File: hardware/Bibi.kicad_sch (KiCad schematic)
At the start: 14 parts, among them M1 Motor_Servo, M2 Motor_Servo, M3 Fan_3pin, U2 Left, U3 Right, U4 GP2Y0A51SK0F

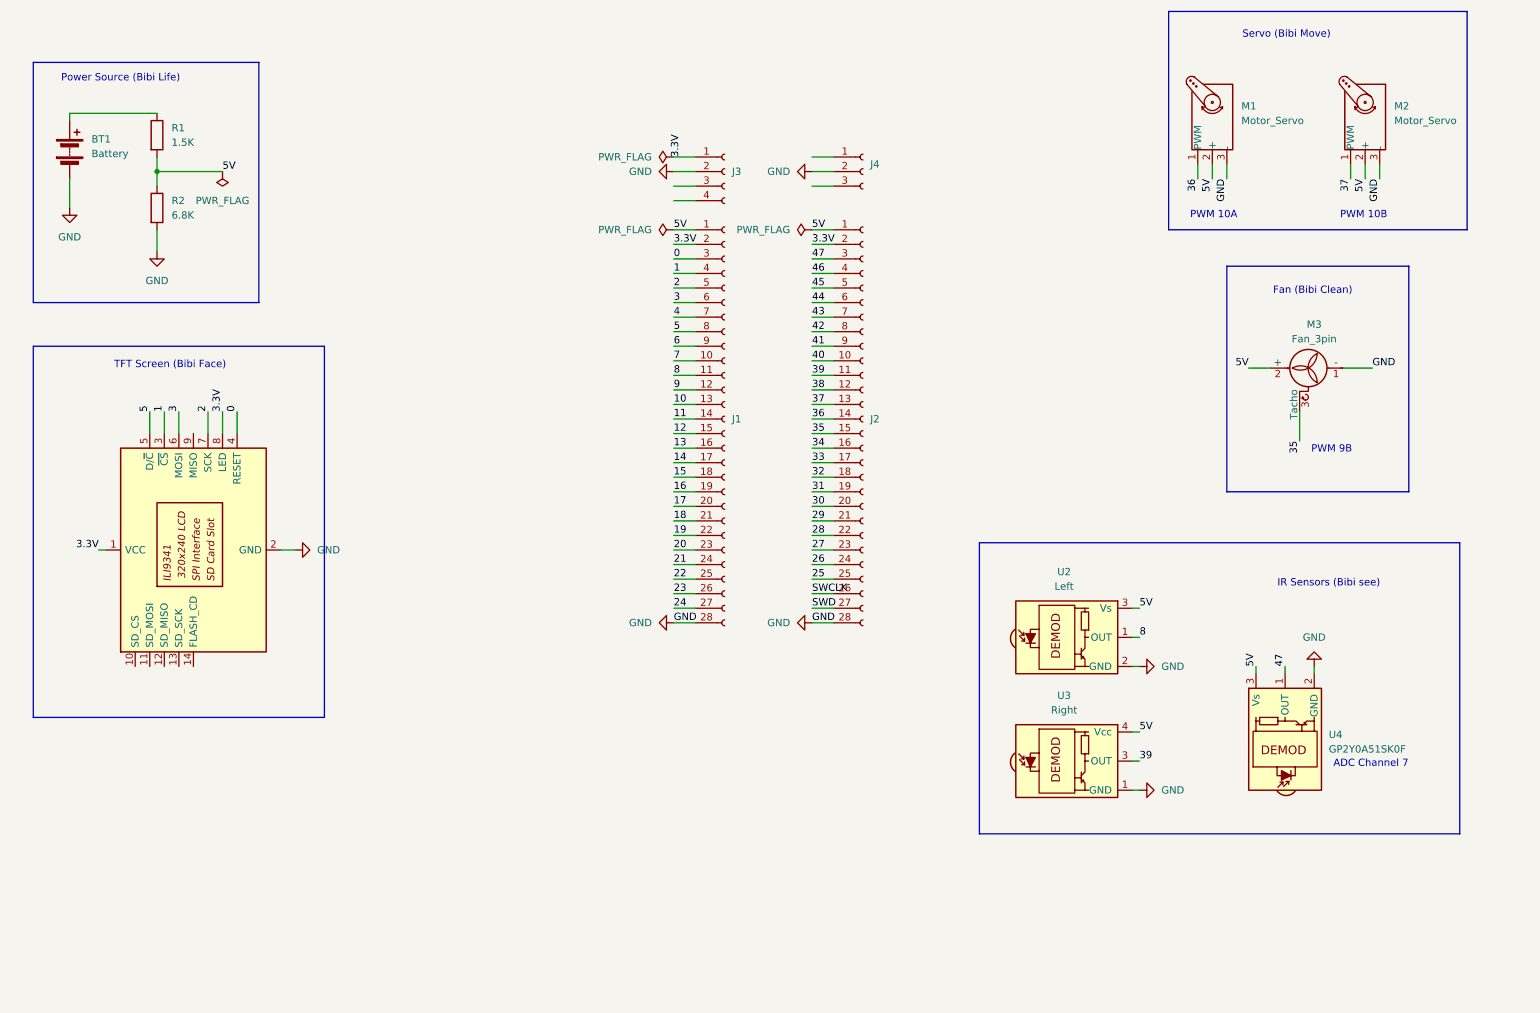
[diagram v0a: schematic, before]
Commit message: updated schematic
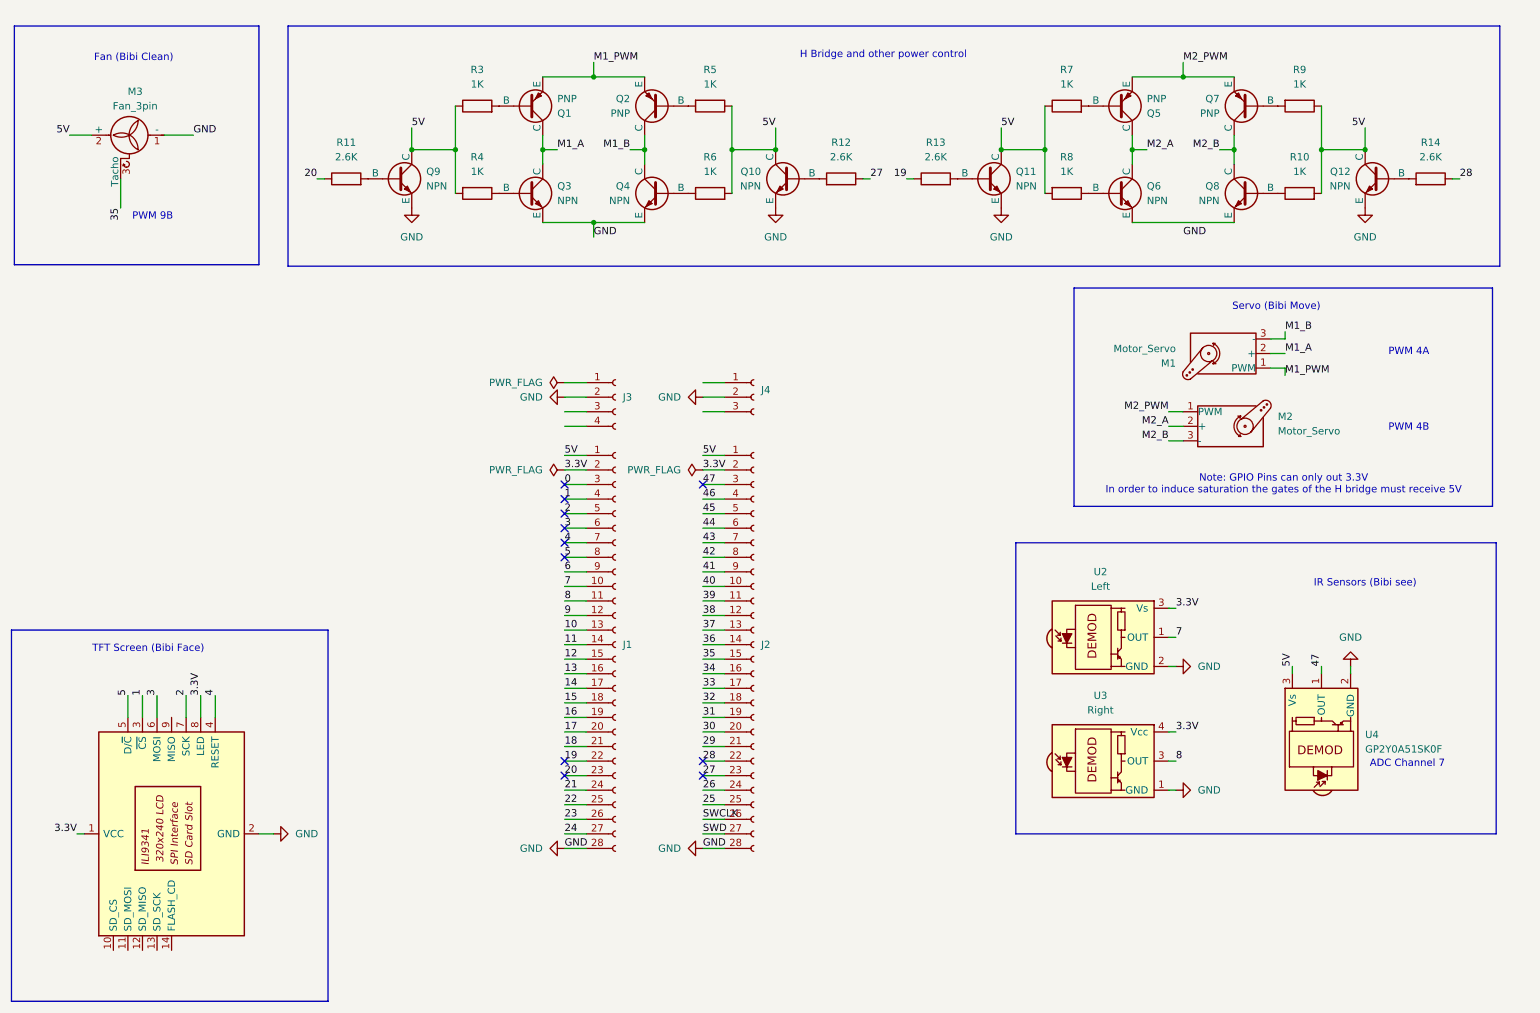
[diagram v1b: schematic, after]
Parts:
- removed BT1: Battery, symbol Device:Battery
- removed R1: 1.5K, Resistor_THT:R_Axial_DIN0411_L9.9mm_D3.6mm_P12.70mm_Horizontal, symbol Device:R
- removed R2: 6.8K, Resistor_THT:R_Axial_DIN0411_L9.9mm_D3.6mm_P12.70mm_Horizontal, symbol Device:R
- added Q1, Q2, Q5, Q7: PNP, symbol Simulation_SPICE:PNP
- added Q10, Q11, Q12, Q3, Q4, Q6, Q8, Q9: NPN, symbol Simulation_SPICE:NPN
- added R10, R3, R4, R5, R6, R7, R8, R9: 1K, symbol Device:R
- added R11, R12, R13, R14: 2.6K, symbol Device:R
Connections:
- net 0: no longer U1.4 (RESET)
- net 19: now also R13.1
- net 20: now also R11.1
- net 27: now also R12.1
- net 28: now also R14.1
- net 3.3V: now also U2.3 (Vs), U3.4 (Vcc); no longer J3.1 (Pin_1)
- net 36: no longer M1.1 (PWM)
- net 37: no longer M2.1 (PWM)
- net 39: no longer U3.3 (OUT)
- net 4: now also U1.4 (RESET)
- net 5V: now also Q10.1 (C), Q11.1 (C), Q12.1 (C), Q9.1 (C), R10.2, R3.1, R4.2, R5.1, R6.2, R7.1, R8.2, R9.1; no longer M1.2 (+), M2.2 (+), U2.3 (Vs), U3.4 (Vcc)
- net 7: now also U2.1 (OUT)
- net 8: now also U3.3 (OUT); no longer U2.1 (OUT)
- net GND: now also Q10.3 (E), Q11.3 (E), Q12.3 (E), Q3.3 (E), Q4.3 (E), Q9.3 (E); no longer M1.3 (-), M2.3 (-)
- new net: Q9.2 (B), R11.2
- new net: Q7.2 (B), R9.2
- new net: Q1.2 (B), R3.2
- new net: Q6.2 (B), R8.1
- new net: Q4.2 (B), R6.1
- new net: Q5.2 (B), R7.2
- new net: Q12.2 (B), R14.2
- new net: Q2.2 (B), R5.2
- new net: Q3.2 (B), R4.1
- new net: Q8.2 (B), R10.1
- new net: Q6.3 (E), Q8.3 (E)
- new net: Q10.2 (B), R12.2
- new net: Q11.2 (B), R13.2
- new net M1_A: M1.2 (+), Q1.1 (C), Q3.1 (C)
- new net M1_B: M1.3 (-), Q2.1 (C), Q4.1 (C)
- new net M1_PWM: M1.1 (PWM), Q1.3 (E), Q2.3 (E)
- new net M2_A: M2.2 (+), Q5.1 (C), Q6.1 (C)
- new net M2_B: M2.3 (-), Q7.1 (C), Q8.1 (C)
- new net M2_PWM: M2.1 (PWM), Q5.3 (E), Q7.3 (E)
- no-connect marks 0 -> 11
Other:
- note added: "H Bridge and other power control"
- note added: "Note: GPIO Pins can only out 3.3V In order to induce saturation the gates of the H bridge must receive 5V"
- note added: "PWM 4A"
- note added: "PWM 4B"
- note removed: "PWM 10A"
- note removed: "PWM 10B"
- note removed: "Power Source (Bibi Life)"
- moved on the sheet: J1, J2, J3, J4, M1, M3, U2, U3, U4
